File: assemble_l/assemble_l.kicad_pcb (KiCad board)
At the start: 2 copper layers, 45 parts, among them J1 Conn_01x02_Pin, SW1 SW_Push, SW10 SW_Push, SW11 SW_Push, SW12 SW_Push, SW13 SW_Push, SW14 SW_Push, SW15 SW_Push, SW16 SW_Push, SW17 SW_Push, SW18 SW_Push, SW19 SW_Push, SW2 SW_Push, SW20 SW_Push, SW21 SW_Push, SW22 SW_Push, SW3 SW_Push, SW4 SW_Push, SW5 SW_Push, SW6 SW_Push, SW7 SW_Push, SW8 SW_Push, SW9 SW_Push, U1 Micon_BLEMicroPro

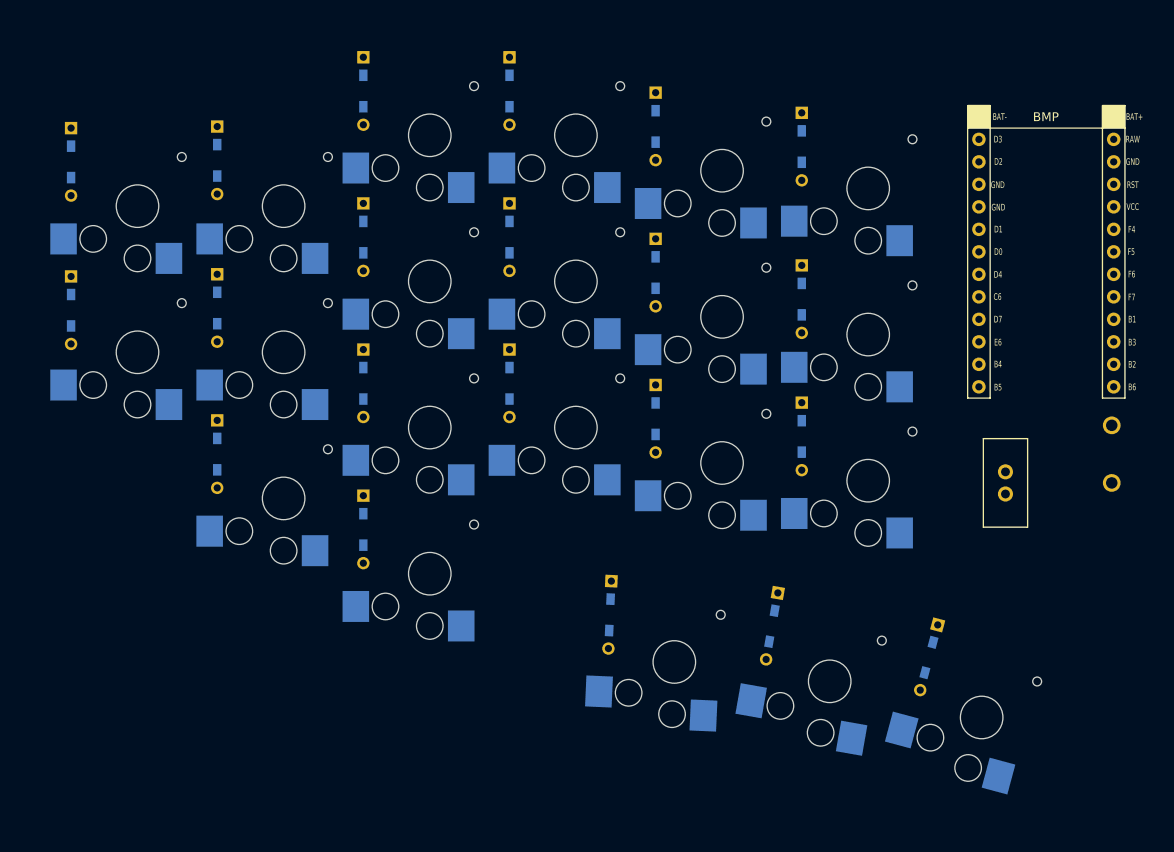
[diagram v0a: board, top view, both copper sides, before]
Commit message: feat: add outline
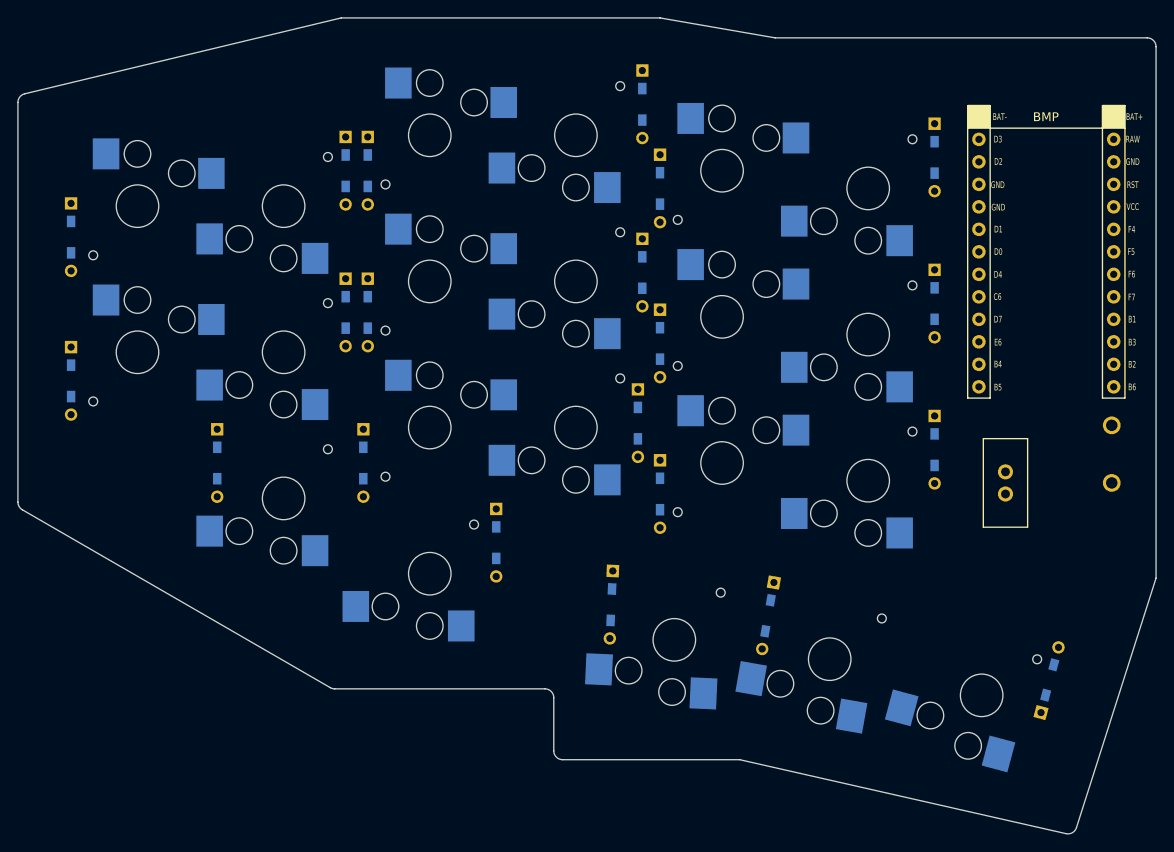
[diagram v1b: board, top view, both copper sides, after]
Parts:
- moved D11 15.5 mm to (125.0, 55.0)
- moved D12 15.2 mm to (124.5, 72.0)
- moved D10 15.1 mm to (125.0, 36.0)
- moved D20 15.1 mm to (158.0, 75.0)
- moved D9 15.1 mm to (108.5, 85.5)
- moved D18 15.0 mm to (158.0, 42.0)
- moved D19 15.0 mm to (158.0, 58.5)
- moved D3 14.5 mm to (91.5, 43.5)
- moved D4 14.5 mm to (91.5, 59.5)
- moved D21 13.9 mm to (171.0, 101.0), turned to 75 degrees
- moved D6 9.01 mm to (94.0, 43.5)
- moved D8 9.00 mm to (93.5, 76.5)
- moved D16 8.51 mm to (127.0, 80.0)
- moved D7 8.51 mm to (94.0, 59.5)
- moved D1 8.50 mm to (60.5, 51.0)
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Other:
- board outline added: 128.5 x 92.1 mm
